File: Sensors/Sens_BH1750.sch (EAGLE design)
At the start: 10 parts, among them IC1 BH1750FVI, X1 VCC, X3 SCL, X4 SDA

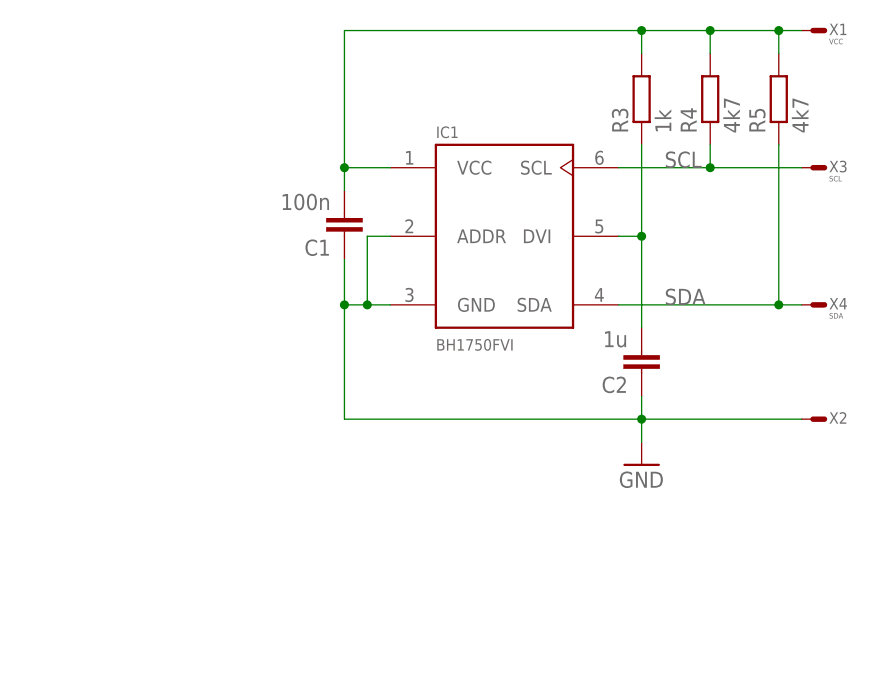
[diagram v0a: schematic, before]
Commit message: Added S4M13
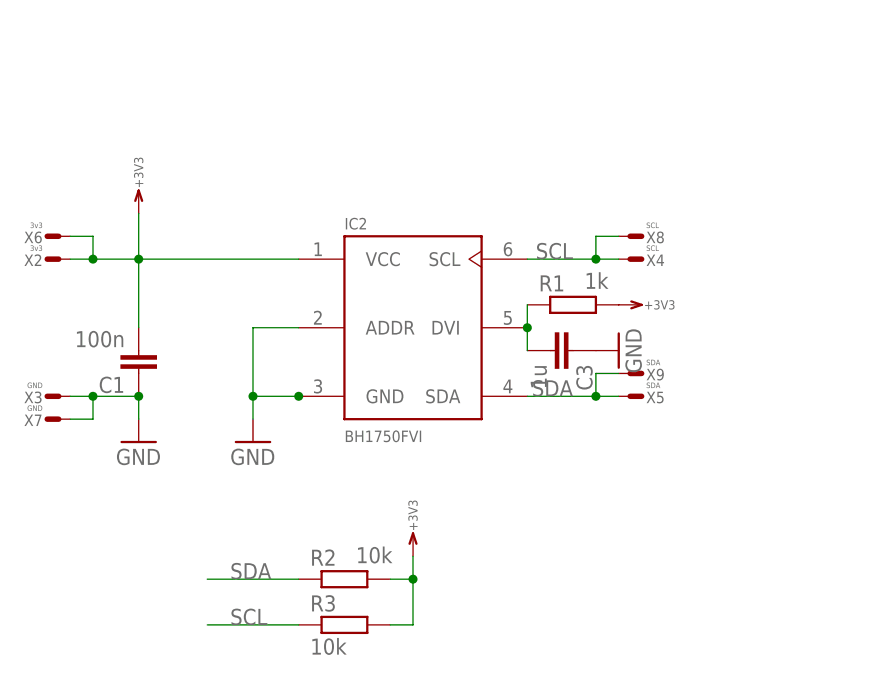
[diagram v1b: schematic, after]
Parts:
- removed C2: 1u, RCL:C0603
- removed IC1: BH1750FVI, Optic:BH1750FVI
- removed R4, R5: 4k7, RCL:R0402
- removed X1: VCC, Conn:WIREPADS2.0/1.0
- added C3: 1u, RCL:C0603
- added IC2: BH1750FVI, Optic:BH1750FVI
- added R1: 1k, RCL:R0603
- added R2: 10k, RCL:R0603
- added X5, X9: SDA, Conn:WIREPADT1.6/0.9
- added X6: 3v3, Conn:WIREPADT1.6/0.9
- added X7: GND, Conn:WIREPADT1.6/0.9
- added X8: SCL, Conn:WIREPADT1.6/0.9
- R3: value 1k -> 10k
- X2: value (none) -> 3v3; device Conn:WIREPADS2.0/1.0 -> Conn:WIREPADT1.6/0.9
- X3: value SCL -> GND; device Conn:WIREPADS2.0/1.0 -> Conn:WIREPADT1.6/0.9
- X4: value SDA -> SCL; device Conn:WIREPADS2.0/1.0 -> Conn:WIREPADT1.6/0.9
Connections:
- removed net N$2: C2.2, IC1.DVI, R3.1
- removed net N$3: C1.2, IC1.VCC, R3.2, R4.2, R5.2, X1.S
- new net +3V3: C1.2, IC2.VCC, R1.2, R2.2, R3.2, X2.S, X6.S
- new net N$1: C3.2, IC2.DVI, R1.1
- net GND: now also C3.1, IC2.ADDR, IC2.GND, X3.S, X7.S; no longer C2.1, IC1.ADDR, IC1.GND, X2.S
- net SCL: now also IC2.SCL, R3.1, X4.S, X8.S; no longer IC1.SCL, R4.1, X3.S
- net SDA: now also IC2.SDA, R2.1, X5.S, X9.S; no longer IC1.SDA, R5.1, X4.S
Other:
- moved on the sheet: C1, R3, X2, X3, X4
